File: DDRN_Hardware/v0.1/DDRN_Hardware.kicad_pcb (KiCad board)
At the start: 2 copper layers, 58.4 x 58.4 mm, 45 parts, among them J2 Conn_Coaxial, J3 Conn_01x02_Pin, J4 Conn_01x04_Pin, J5 Conn_01x06_Pin, J8 Conn_02x05_Top_Bottom, Q1 BSS119, Q2 BSS119, SW1 SW_Push, U1 LoRa-E5, U2 MAX1932, U3 BMP390L, U4 W25Q32JVSS, U5 LSM303AGR, U6 AP2112K-3.3

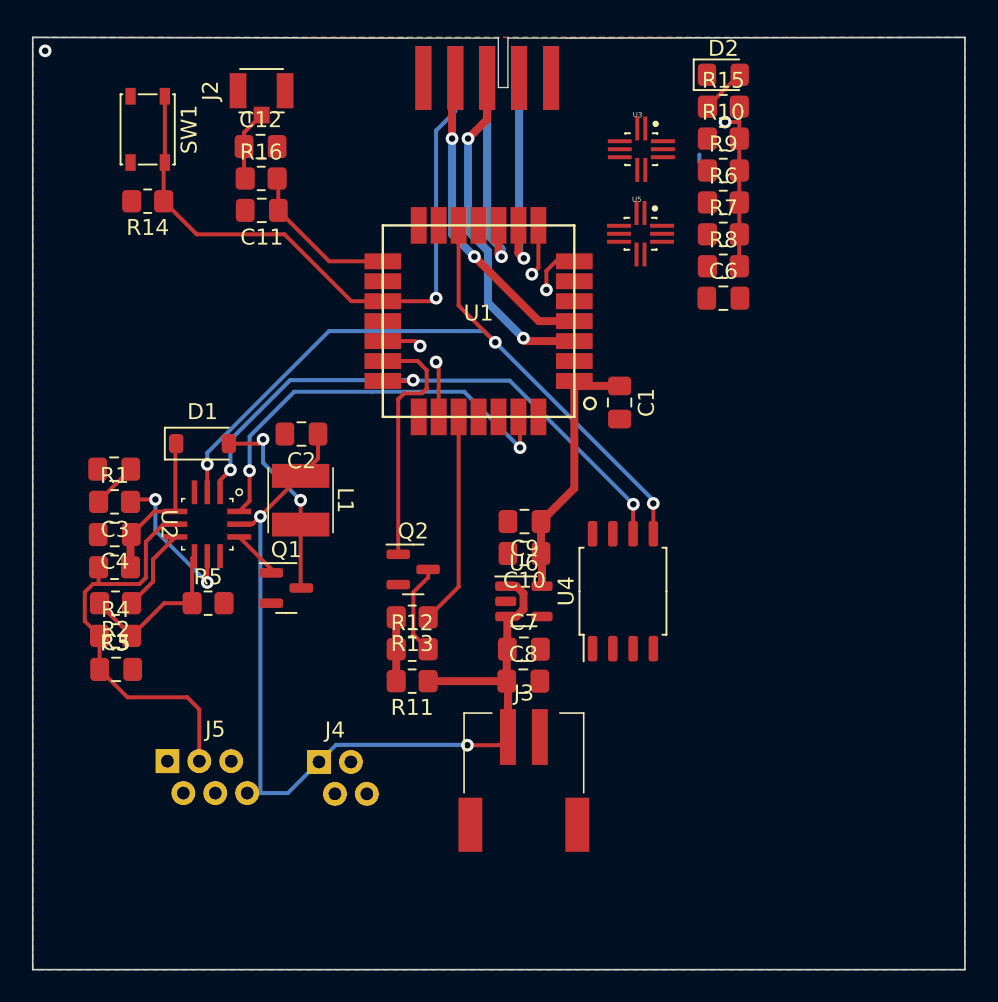
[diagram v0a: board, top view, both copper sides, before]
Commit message: v0.1 pcb complete?
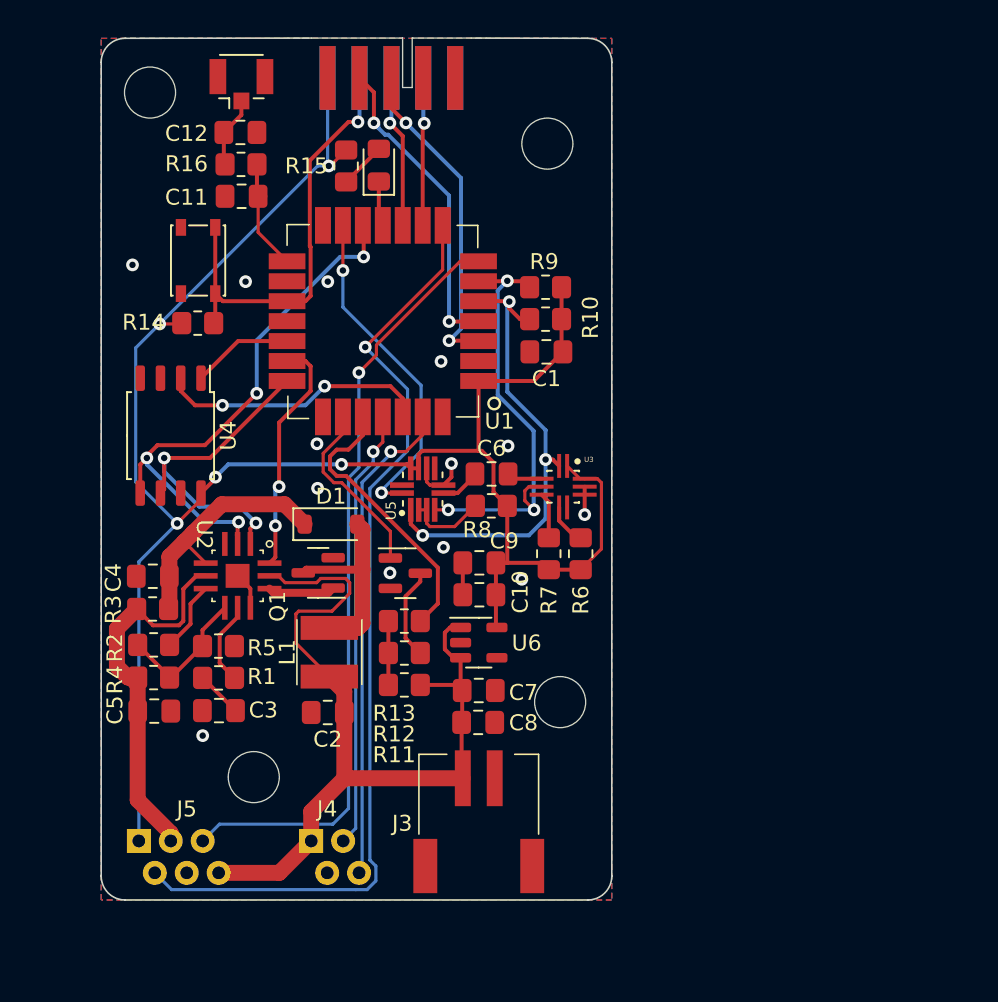
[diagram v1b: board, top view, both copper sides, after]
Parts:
- added H1: MountingHole, MountingHole:MountingHole_3.2mm_M3_DIN965, F.Cu at (82.1, 98.0)
- added H2: MountingHole, MountingHole:MountingHole_3.2mm_M3_DIN965, F.Cu at (57.2, 94.8)
- added H3: MountingHole, MountingHole:MountingHole_3.2mm_M3_DIN965, F.Cu at (82.9, 133.1)
- added H4: MountingHole, MountingHole:MountingHole_3.2mm_M3_DIN965, F.Cu at (63.7, 137.8)
- U5: footprint Library:bmp390_handsolder -> Library:lsm303_handsolder
- moved U4 30.0 mm to (58.5, 116.3), turned to -90 degrees
- moved R15 23.9 mm to (69.5, 99.5), turned to 90 degrees
- moved R6 23.8 mm to (84.2, 123.8), turned to -90 degrees
- moved R7 22.8 mm to (82.2, 123.8), turned to -90 degrees
- moved D2 22.3 mm to (71.5, 99.4), turned to 90 degrees
- moved U3 21.7 mm to (83.0, 119.5)
- moved U5 21.0 mm to (74.2, 119.7), turned to 90 degrees
- moved R8 20.9 mm to (78.5, 120.8)
- moved C6 18.2 mm to (78.6, 118.8)
- moved C2 17.5 mm to (68.3, 133.7)
- moved C3 16.5 mm to (61.5, 133.6)
- moved R10 14.5 mm to (82.0, 107.0)
- moved R9 14.5 mm to (82.0, 109.0)
- moved R1 12.8 mm to (61.5, 131.5)
- moved L1 9.69 mm to (68.4, 129.9), turned to 90 degrees
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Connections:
- U1 pad 18: /Bias_Enable -> unconnected-(U1-PA3-Pad18)
- U1 pad 19: /Stim_Enable -> /Memory_CS
- U1 pad 20: /Battery_Monitor_Enable -> /Bias_CS
- U1 pad 23: /Anneal_Enable -> /Battery_Monitor_Enable
- U1 pad 25: /Memory_CS -> /Stim_Enable
- U1 pad 27: /Bias_CS -> /Anneal_Enable
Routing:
- net /3v3: track 27.6 -> 120.6 mm, vias 1 -> 5
- net /SiPM_Temp: track 3.23 -> 59.8 mm
- net /SiPM_Signal: track 3.19 -> 48.5 mm
- net /SCL: track 0.00 -> 29.6 mm, vias 0 -> 3
- net /Anneal_Enable: track 3.51 -> 30.8 mm
- net /SDA: track 0.50 -> 27.7 mm, vias 0 -> 3
- net /Stim_Enable: track 2.47 -> 27.6 mm
- net /ACCEL_INT: track 0.00 -> 21.1 mm, vias 0 -> 2
- net /MISO: track 0.00 -> 17.1 mm, vias 0 -> 2
- net /SCK: track 37.4 -> 21.4 mm, vias 3 -> 2
- net /MOSI: track 48.4 -> 34.3 mm, vias 3 -> 4
- net /RST: track 40.7 -> 27.7 mm
- net GND: track 0.00 -> 11.6 mm, vias 1 -> 13
- net /Bias_CS: track 26.5 -> 15.0 mm
- net /Memory_CS: track 0.00 -> 6.36 mm
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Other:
- board size 58.4 x 58.4 mm -> 32 x 54 mm
